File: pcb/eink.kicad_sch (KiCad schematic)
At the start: 28 parts, among them J1 USB_C_Receptacle_USB2.0_16P, J3 E-paper Display, SW1 SW_Push, SW2 RotaryEncoder_Switch, U1 ESP-12F, U3 RT6150AGQW, U4 CH340N

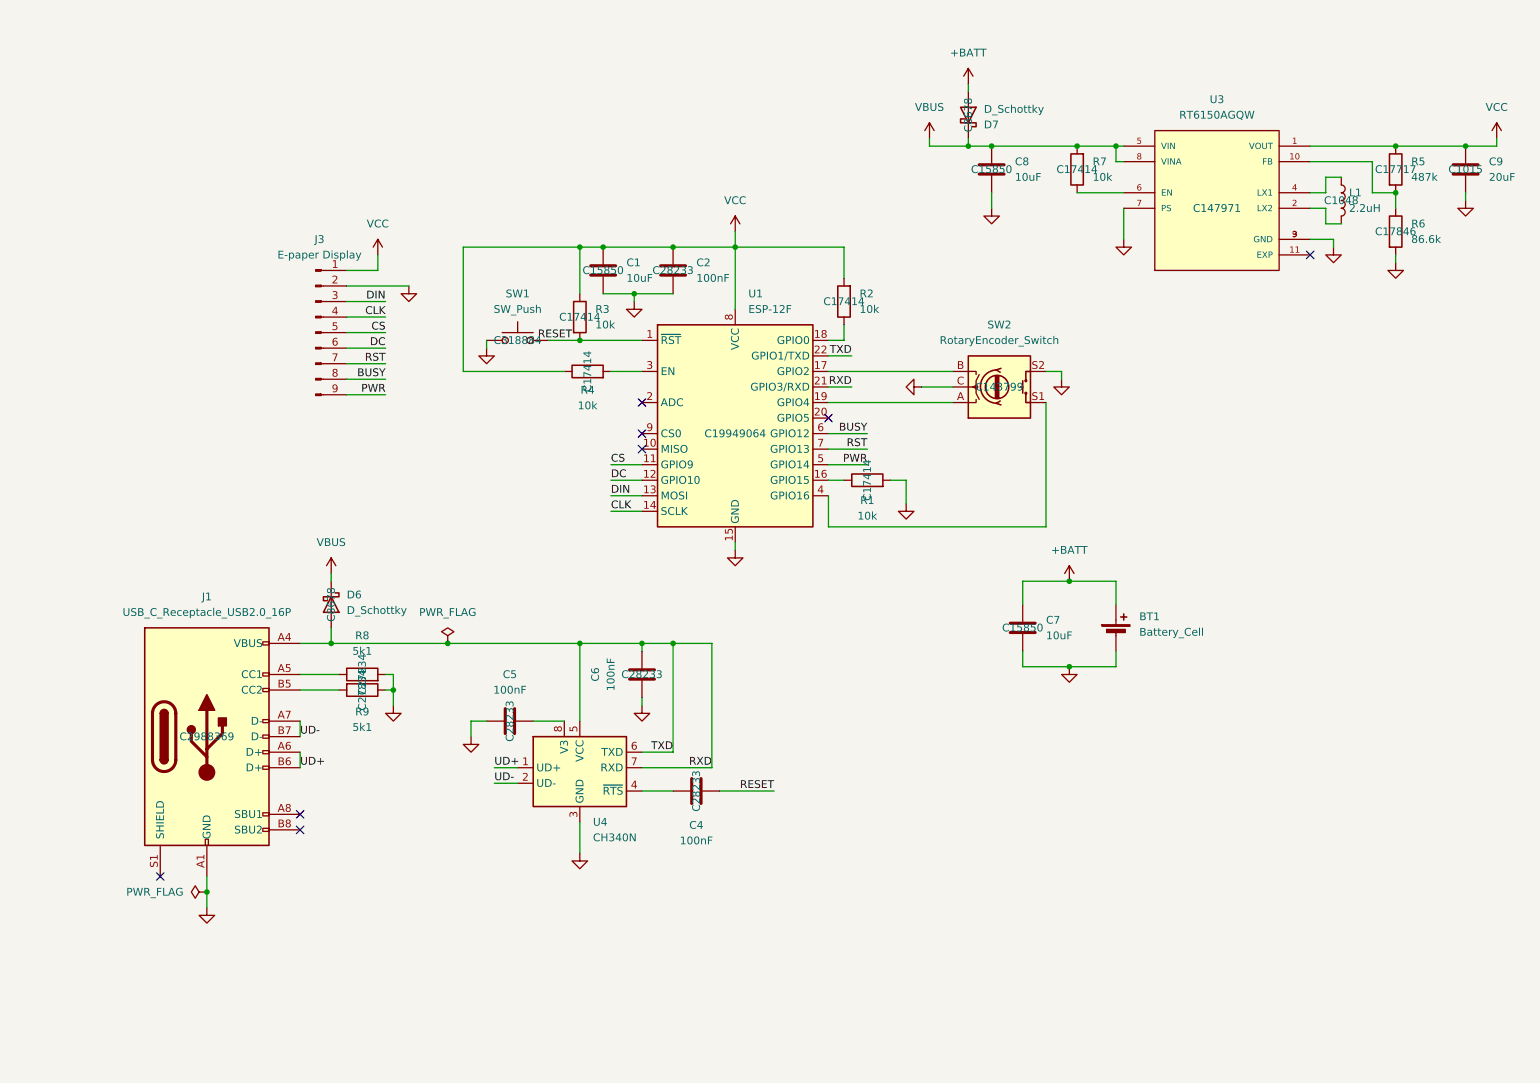
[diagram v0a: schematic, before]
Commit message: pcb
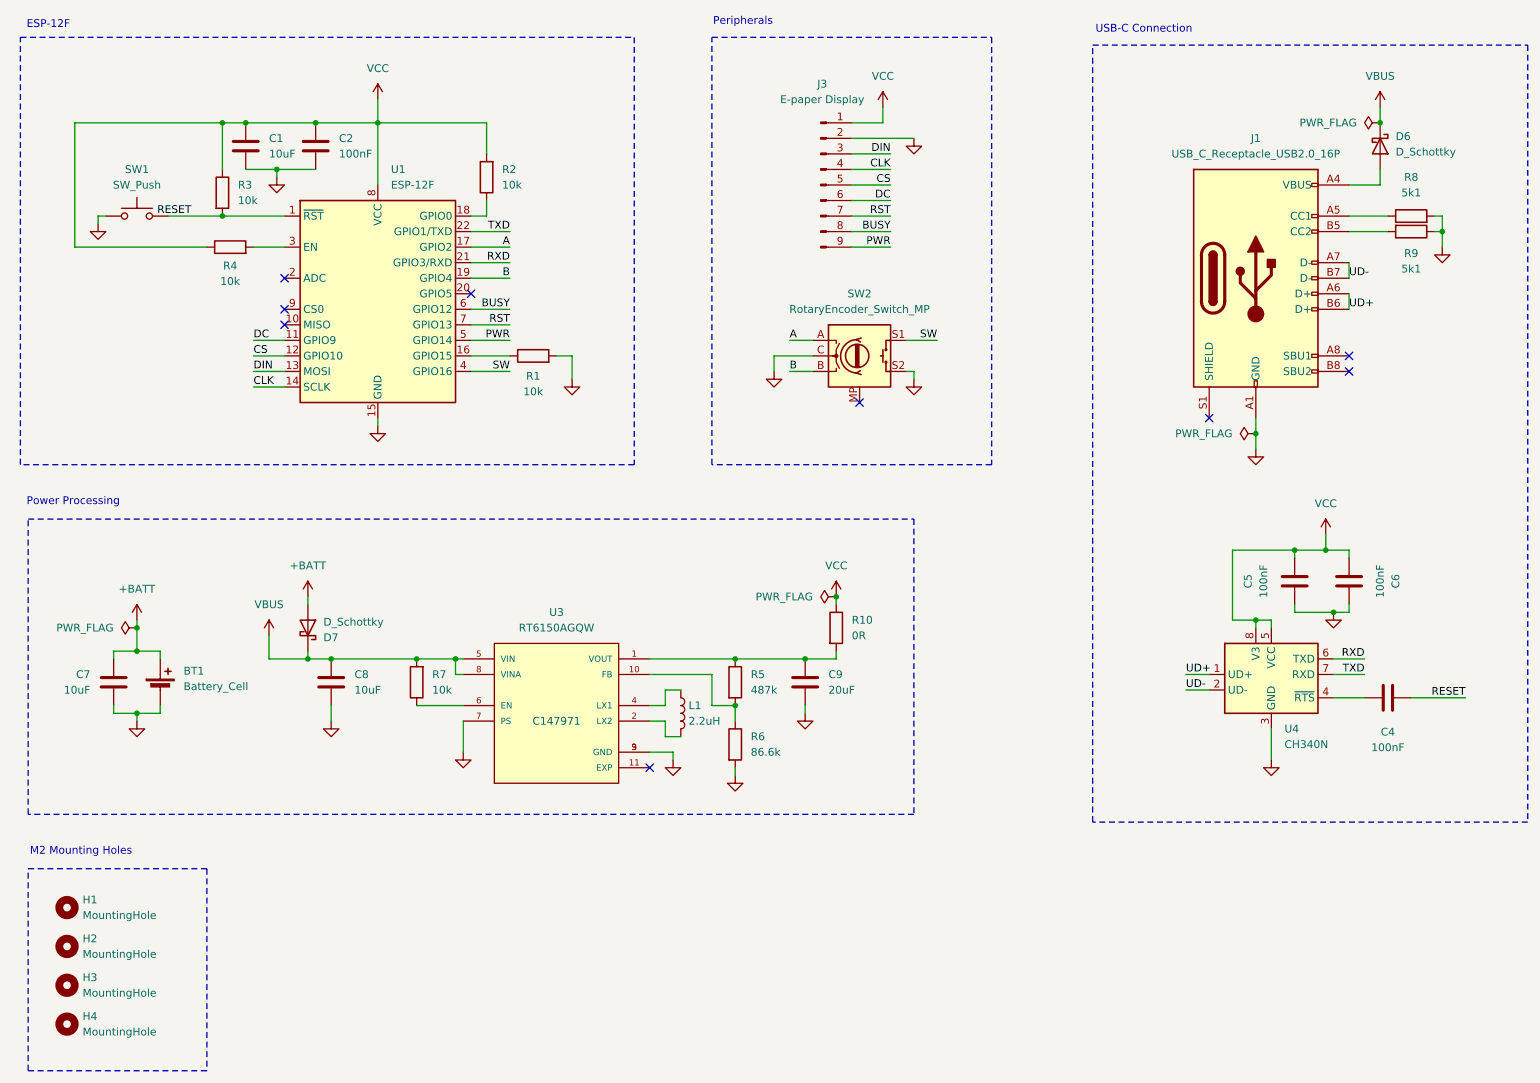
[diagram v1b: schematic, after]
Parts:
- removed SW2: RotaryEncoder_Switch, Rotary_Encoder:RotaryEncoder_Bourns_Vertical_PEC12R-3x17F-Sxxxx, symbol Device:RotaryEncoder_Switch
- added H1, H2, H3, H4: MountingHole, MountingHole:MountingHole_2.2mm_M2, symbol Mechanical:MountingHole
- added R10: 0R, symbol Device:R
- added SW2: RotaryEncoder_Switch_MP, custom:EC11J, symbol Device:RotaryEncoder_Switch_MP
- R5, R6: footprint Capacitor_SMD:C_0805_2012Metric -> Resistor_SMD:R_0805_2012Metric
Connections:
- net CS: now also U1.12 (GPIO10); no longer U1.11 (GPIO9)
- net DC: now also U1.11 (GPIO9); no longer U1.12 (GPIO10)
- net GND: now also SW2.C, SW2.S2
- net RXD: no longer C6.1, D6.2 (A), J1.A4 (VBUS), J1.A9 (VBUS), J1.B4 (VBUS), J1.B9 (VBUS), U1.22 (GPIO1/TXD), U4.5 (VCC), U4.7 (RXD)
- net VCC: now also C5.1, C6.1, U4.5 (VCC), U4.8 (V3), R10.1; no longer C9.1, R5.1, U3.1 (VOUT)
- net B: now reaches U1.19 (GPIO4)
- net B: now also SW2.B
- net A: now reaches U1.17 (GPIO2)
- net A: now also SW2.A
- net SW: now reaches U1.4 (GPIO16)
- net SW: now also SW2.S1
- new net: D6.2 (A), J1.A4 (VBUS), J1.A9 (VBUS), J1.B4 (VBUS), J1.B9 (VBUS)
- new net: C9.1, R10.2, R5.1, U3.1 (VOUT)
- new net TXD: U1.22 (GPIO1/TXD), U4.7 (RXD)
- no-connect marks 8 -> 9
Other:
- note added: "ESP-12F"
- note added: "M2 Mounting Holes"
- note added: "Peripherals"
- note added: "Power Processing"
- note added: "USB-C Connection"
- moved on the sheet: BT1, C1, C2, C4, C5, C6, C7, C8, C9, D6, D7, J1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
